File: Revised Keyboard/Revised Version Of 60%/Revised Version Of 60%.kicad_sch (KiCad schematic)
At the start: 102 parts, among them J1 AVR-ISP-6, SW1 SW_Push, U1 AT90USB1286-A, U2 PRTR5V0U2X, Y1 Crystal_GND24_Small

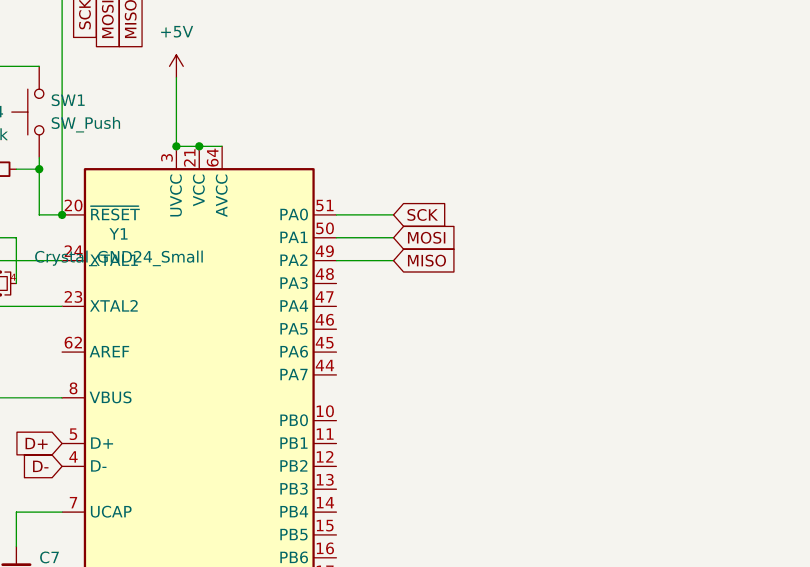
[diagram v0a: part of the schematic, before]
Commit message: Update
General Update of files
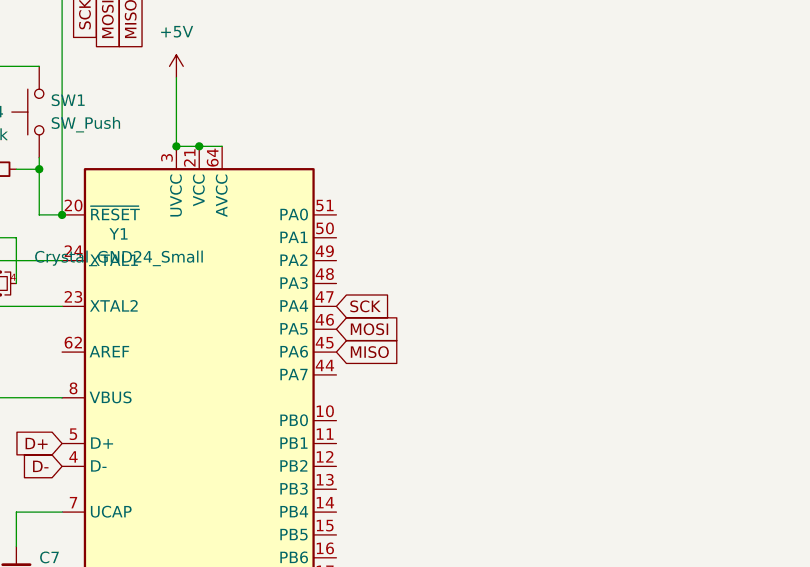
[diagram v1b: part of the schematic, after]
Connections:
- net MISO: now also U1.45 (PA6); no longer U1.49 (PA2)
- net MOSI: now also U1.46 (PA5); no longer U1.50 (PA1)
- net SCK: now also U1.47 (PA4); no longer U1.51 (PA0)
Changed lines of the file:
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@@
-    (stroke (width 0) (type default) (color 0 0 0 0))
-  )
-  (wire (pts (xy 121.92 58.42) (xy 128.27 58.42))
     (stroke (width 0) (type default) (color 0 0 0 0))
   )
@@
     (stroke (width 0) (type default) (color 0 0 0 0))
   )
-  (wire (pts (xy 121.92 55.88) (xy 128.27 55.88))
-    (stroke (width 0) (type default) (color 0 0 0 0))
-  )
   (wire (pts (xy 233.68 85.09) (xy 240.03 85.09))
     (stroke (width 0) (type default) (color 0 0 0 0))
@@
     (stroke (width 0) (type default) (color 0 0 0 0))
   )
-  (wire (pts (xy 121.92 53.34) (xy 128.27 53.34))
-    (stroke (width 0) (type default) (color 0 0 0 0))
-  )
   (wire (pts (xy 252.73 90.17) (xy 254 90.17))
     (stroke (width 0) (type default) (color 0 0 0 0))
@@
     (stroke (width 0) (type default) (color 0 0 0 0))
   )
-  (global_label "MOSI" (shape input) (at 128.27 55.88 0) (fields_autoplaced)
+  (global_label "MOSI" (shape input) (at 121.92 66.04 0) (fields_autoplaced)
     (effects (font (size 1.27 1.27)) (justify left))
-    (property "Intersheet References" "${INTERSHEET_REFS}" (id 0) (at 135.2793 55.9594 0)
+    (property "Intersheet References" "${INTERSHEET_REFS}" (id 0) (at 128.9293 66.1194 0)
       (effects (font (size 1.27 1.27)) (justify left) hide)
     )
@@
     )
   )
-  (global_label "SCK" (shape input) (at 128.27 53.34 0) (fields_autoplaced)
+  (global_label "SCK" (shape input) (at 121.92 63.5 0) (fields_autoplaced)
     (effects (font (size 1.27 1.27)) (justify left))
-    (property "Intersheet References" "${INTERSHEET_REFS}" (id 0) (at 134.4326 53.4194 0)
+    (property "Intersheet References" "${INTERSHEET_REFS}" (id 0) (at 128.0826 63.5794 0)
       (effects (font (size 1.27 1.27)) (justify left) hide)
     )
@@
     )
   )
-  (global_label "MISO" (shape input) (at 128.27 58.42 0) (fields_autoplaced)
+  (global_label "MISO" (shape input) (at 121.92 68.58 0) (fields_autoplaced)
     (effects (font (size 1.27 1.27)) (justify left))
-    (property "Intersheet References" "${INTERSHEET_REFS}" (id 0) (at 135.2793 58.4994 0)
+    (property "Intersheet References" "${INTERSHEET_REFS}" (id 0) (at 128.9293 68.6594 0)
       (effects (font (size 1.27 1.27)) (justify left) hide)
     )
